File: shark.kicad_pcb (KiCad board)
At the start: 2 copper layers, 225.6 x 74.8 mm, 259 parts, among them J1 USB_C_Receptacle, Q1 AO4406AL, SW1 MXSwitch, SW10 MXSwitch, SW11 MXSwitch, SW12 MXSwitch, SW13 MXSwitch, SW14 MXSwitch, SW15 MXSwitch, SW16 MXSwitch, SW17 MXSwitch, SW18 MXSwitch, SW19 MXSwitch, SW2 MXSwitch, SW20 MXSwitch, SW21 MXSwitch, SW22 MXSwitch, SW23 MXSwitch, SW24 MXSwitch, SW25 MXSwitch, SW26 MXSwitch, SW27 MXSwitch, SW28 MXSwitch, SW29 MXSwitch, SW3 MXSwitch, SW30 MXSwitch, SW31 MXSwitch, SW32 MXSwitch, SW33 MXSwitch, SW34 MXSwitch, SW35 MXSwitch, SW36 MXSwitch, SW37 MXSwitch, SW38 MXSwitch, SW39 MXSwitch, SW4 MXSwitch, SW40 MXSwitch, SW41 MXSwitch, SW42 MXSwitch, SW43 MXSwitch, SW44 MXSwitch, SW45 MXSwitch, SW46 MXSwitch, SW47 MXSwitch, SW48 MXSwitch, SW49 MXSwitch, SW5 MXSwitch, SW50 MXSwitch, SW51 MXSwitch, SW6 MXSwitch, SW7 MXSwitch, SW8 MXSwitch, SW9 MXSwitch, U1 STM32F303CCT7, U2 MCP1700-3302E_SOT23, Y1 8MHz

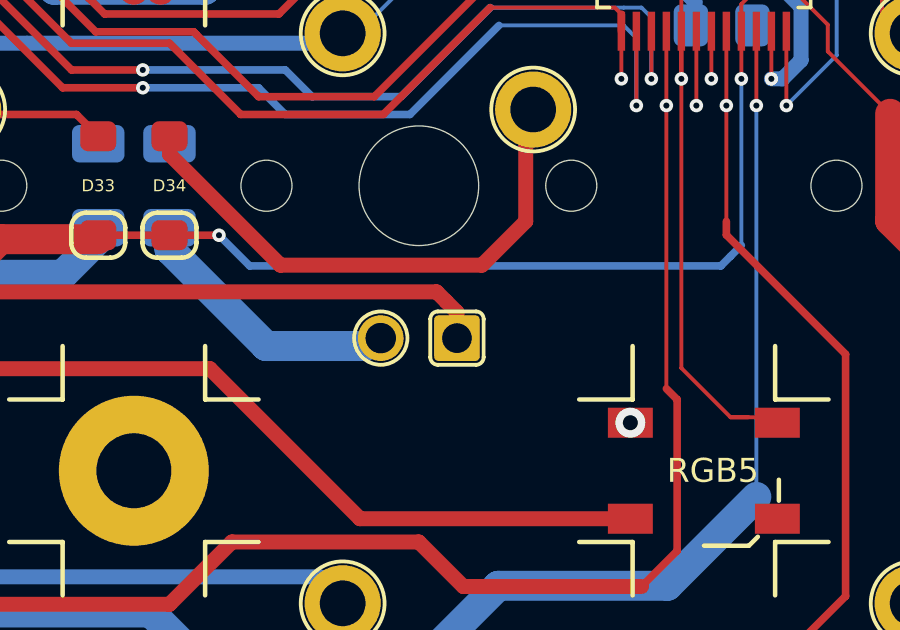
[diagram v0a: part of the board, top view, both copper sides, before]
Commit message: Edited gerbers
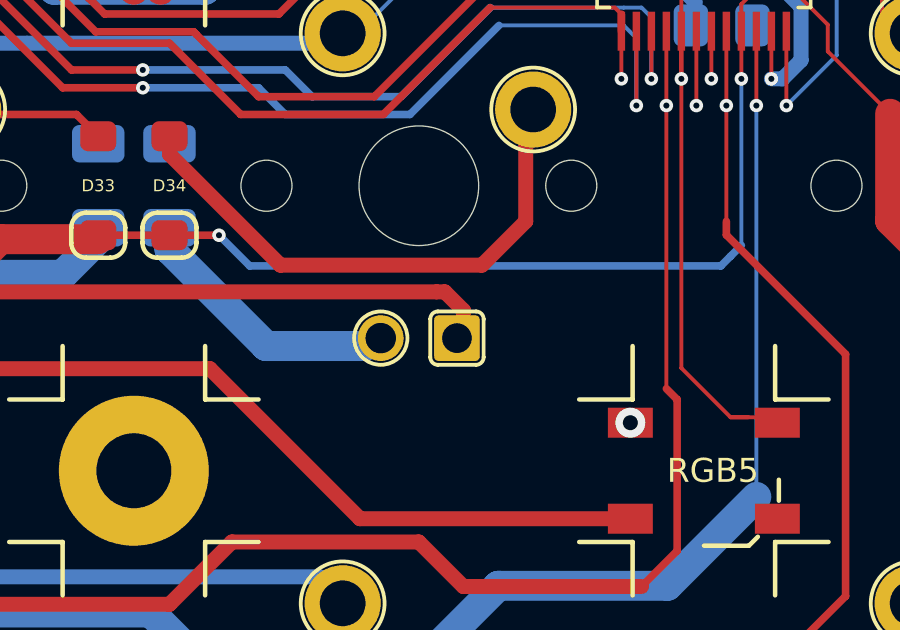
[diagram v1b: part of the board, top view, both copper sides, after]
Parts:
- removed the Y1 at (207.2, 102.4) (x2)
- added Y1 (x2): 8MHz, crystal:Crystal_SMD_5032-4Pin_5.0x3.2mm, F.Cu at (207.2, 102.4)
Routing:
- net Net-(LED1-PadK): track 1132.7 -> 1131.8 mm
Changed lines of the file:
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@@
     (thickness 1.6)
     (drawings 440)
-    (tracks 1809)
+    (tracks 1808)
     (zones 0)
     (modules 259)
@@
   (segment (start 64.1505 78.696125) (end 64.1505 78.993) (width 0.254) (layer F.Cu) (net 72) (status 30))
   (segment (start 197.1505 115.8055) (end 197.1505 116.696125) (width 0.5) (layer F.Cu) (net 72) (status 20))
-  (segment (start 216.233 117.323) (end 216.233 116.461) (width 0.5) (layer F.Cu) (net 72) (status 10))
   (segment (start 159.1505 116.993) (end 158.853625 116.993) (width 0.254) (layer F.Cu) (net 72) (status 30))
   (segment (start 235.233 117.323) (end 246.168 117.323) (width 1) (layer F.Cu) (net 72) (status 10))
@@
   (segment (start 121.12233 104.676825) (end 121.12233 100.990575) (width 1) (layer B.Cu) (net 72) (status 30))
   (via (at 121.39108 104.676825) (size 1) (drill 0.5) (layers F.Cu B.Cu) (net 72) (status 30))
-  (segment (start 216.233 117.323) (end 216.233 116.461) (width 0.254) (layer B.Cu) (net 72) (status 10))
   (segment (start 245.24425 131.243) (end 241.68175 131.243) (width 0.254) (layer F.Cu) (net 72))
   (segment (start 241.68175 131.243) (end 239.30675 133.618) (width 0.254) (layer F.Cu) (net 72))
@@
   (segment (start 135.4005 99.77425) (end 139.853625 99.77425) (width 0.7) (layer F.Cu) (net 72))
   (segment (start 133.94925 98.323) (end 135.4005 99.77425) (width 0.7) (layer F.Cu) (net 72))
-  (segment (start 216.233 116.461) (end 215.874375 116.102375) (width 0.5) (layer F.Cu) (net 72))
   (segment (start 159.1505 115.78125) (end 159.1505 117.289875) (width 0.5) (layer F.Cu) (net 72) (status 20))
   (segment (start 141.882 115.78125) (end 159.1505 115.78125) (width 0.5) (layer F.Cu) (net 72))
@@
   (segment (start 65.021073 137.111073) (end 65.021073 137.136198) (width 0.254) (layer F.Cu) (net 72))
   (segment (start 85.228625 100.071125) (end 102.125 100.071125) (width 0.7) (layer F.Cu) (net 72))
-  (segment (start 215.55325 115.78125) (end 215.874375 116.102375) (width 0.5) (layer F.Cu) (net 72))
   (segment (start 120.259875 100.071125) (end 121.1505 99.1805) (width 0.7) (layer F.Cu) (net 72))
   (segment (start 178.233 117.34747) (end 178.233 115.80572) (width 0.5) (layer F.Cu) (net 72))
   (segment (start 159.1505 115.78125) (end 178.233 115.78125) (width 0.5) (layer F.Cu) (net 72))
   (segment (start 178.233 115.78125) (end 215.55325 115.78125) (width 0.5) (layer F.Cu) (net 72))
+  (segment (start 215.55325 115.78125) (end 215.83029 115.78125) (width 0.5) (layer F.Cu) (net 72))
+  (segment (start 215.83029 115.78125) (end 216.44852 116.39948) (width 0.5) (layer F.Cu) (net 72))
+  (segment (start 216.44852 116.39948) (end 216.44852 116.99324) (width 0.5) (layer F.Cu) (net 72))
   (segment (start 55.24425 76.368) (end 58.463 79.58675) (width 1) (layer B.Cu) (net 73))
   (segment (start 55.24425 75.643) (end 55.24425 76.368) (width 1) (layer B.Cu) (net 73) (status 10))

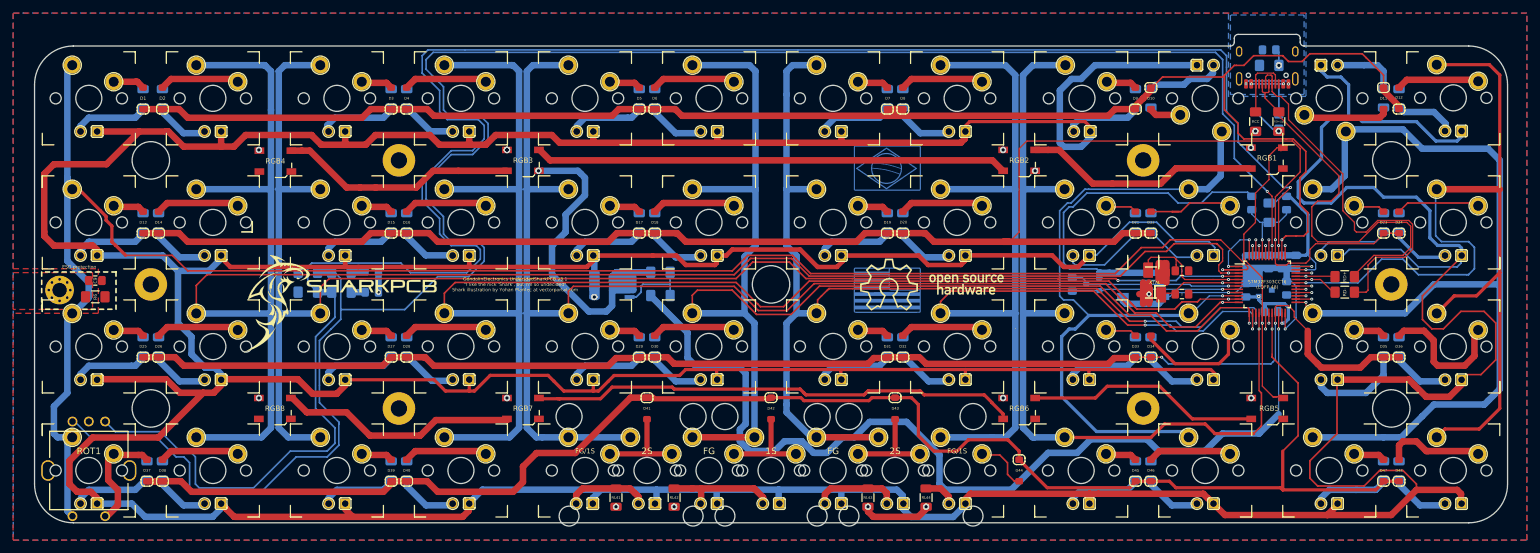
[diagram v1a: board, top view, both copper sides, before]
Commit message: Fixed little problem with edge cuts
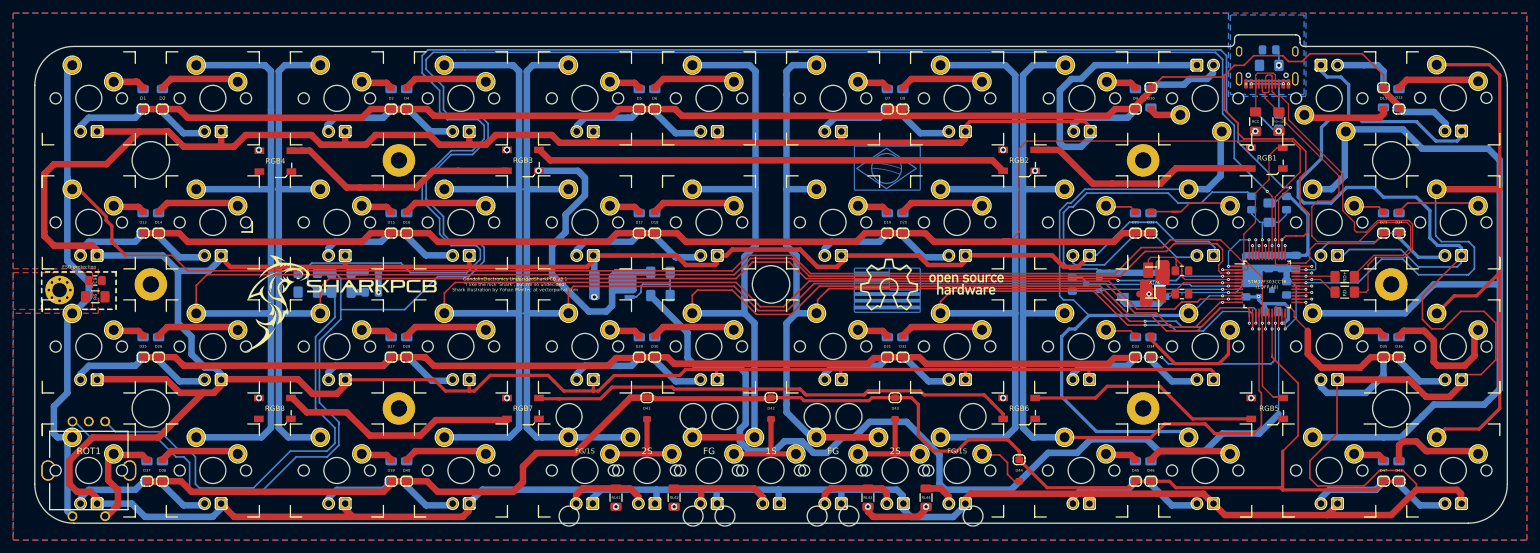
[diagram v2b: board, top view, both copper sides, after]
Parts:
- removed the Y1 at (207.2, 102.4) (x2)
- added Y1 (x2): 8MHz, crystal:Crystal_SMD_5032-4Pin_5.0x3.2mm, F.Cu at (207.2, 102.4)
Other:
- outline, holes or cut-outs redrawn
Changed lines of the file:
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@@
   (title_block
     (title SharkPCB)
-    (date 2019-02-20)
-    (rev V3.1)
+    (date 2019-02-27)
+    (rev V3.1.1)
     (company "Gondolin Electronics")
   )
@@
     )
   )
+  (gr_arc (start 255.27 72.263) (end 261.239 72.263) (angle -90) (layer Edge.Cuts) (width 0.15))
+  (gr_arc (start 230.124 65.659) (end 229.489 65.659) (angle -90) (layer Edge.Cuts) (width 0.15))
+  (gr_arc (start 228.854 65.151) (end 229.489 65.151) (angle -90) (layer Edge.Cuts) (width 0.15))
+  (gr_arc (start 220.091 65.151) (end 220.091 64.516) (angle -90) (layer Edge.Cuts) (width 0.15))
+  (gr_arc (start 218.821 65.659) (end 218.821 66.294) (angle -90) (layer Edge.Cuts) (width 0.15))
+  (gr_arc (start 41.656 72.263) (end 41.656 66.294) (angle -90) (layer Edge.Cuts) (width 0.15))
+  (gr_arc (start 41.656 133.35) (end 35.687 133.35) (angle -90) (layer Edge.Cuts) (width 0.15))
   (gr_text FG/1S (at 176.963 128.27425) (layer F.SilkS)
     (effects (font (size 0.75 0.75) (thickness 0.1875)))
@@
     (effects (font (size 0.8 0.8) (thickness 0.2)) (justify mirror))
   )
-  (gr_arc (start 41.588 72.164751) (end 41.588 66.227251) (angle -90) (layer Edge.Cuts) (width 0.15))
-  (gr_arc (start 41.588 133.321125) (end 35.6505 133.321125) (angle -90) (layer Edge.Cuts) (width 0.15))
-  (gr_arc (start 255.338 133.321125) (end 255.338 139.258625) (angle -90) (layer Edge.Cuts) (width 0.15))
-  (gr_arc (start 255.338 72.164875) (end 261.2755 72.164875) (angle -90) (layer Edge.Cuts) (width 0.15))
+  (gr_arc (start 255.27 133.35) (end 255.27 139.319) (angle -90) (layer Edge.Cuts) (width 0.15))
   (gr_circle (center 243.46332 121.743064) (end 246.330134 121.743064) (layer Edge.Cuts) (width 0.15))
   (gr_circle (center 243.46332 83.742936) (end 246.330134 83.742936) (layer Edge.Cuts) (width 0.15))
@@
   (gr_line (start 49.30675 67.118) (end 51.088 67.118) (layer F.SilkS) (width 0.15))
   (gr_line (start 51.088 67.118) (end 51.088 68.89925) (layer F.SilkS) (width 0.15))
-  (gr_line (start 220.009875 64.446125) (end 228.916396 64.445995) (layer Edge.Cuts) (width 0.15))
-  (gr_line (start 219.416125 65.633625) (end 219.416125 65.039875) (layer Edge.Cuts) (width 0.15))
-  (gr_arc (start 228.916398 65.039747) (end 229.510148 65.039747) (angle -90) (layer Edge.Cuts) (width 0.15))
-  (gr_arc (start 230.103623 65.633625) (end 229.509873 65.633625) (angle -90) (layer Edge.Cuts) (width 0.15))
-  (gr_arc (start 220.009875 65.039875) (end 220.009875 64.446125) (angle -90) (layer Edge.Cuts) (width 0.15))
-  (gr_arc (start 218.822612 65.633501) (end 218.822612 66.227251) (angle -90) (layer Edge.Cuts) (width 0.15))
+  (gr_line (start 220.091 64.516) (end 228.854 64.516) (layer Edge.Cuts) (width 0.15))
+  (gr_line (start 219.456 65.659) (end 219.456 65.151) (layer Edge.Cuts) (width 0.15))
   (gr_line (start 68.988926 93.118786) (end 68.988926 94.706286) (layer F.SilkS) (width 0.254))
   (gr_line (start 68.988926 94.706286) (end 67.401426 94.706286) (layer F.SilkS) (width 0.254))
-  (gr_line (start 229.509873 65.633625) (end 229.509873 65.039875) (layer Edge.Cuts) (width 0.15))
+  (gr_line (start 229.489 65.659) (end 229.489 65.151) (layer Edge.Cuts) (width 0.15))
   (gr_text "Surge\nprotection" (at 224.463 81.96175) (layer B.SilkS)
     (effects (font (size 0.508 0.508) (thickness 0.127)) (justify mirror))
@@
     (effects (font (size 0.508 0.508) (thickness 0.0762)))
   )
-  (gr_line (start 35.6505 133.321125) (end 35.6505 72.164875) (layer Edge.Cuts) (width 0.15))
-  (gr_line (start 255.338 139.258625) (end 41.588 139.258625) (layer Edge.Cuts) (width 0.15))
-  (gr_line (start 261.2755 72.164875) (end 261.2755 133.321125) (layer Edge.Cuts) (width 0.15))
+  (gr_line (start 35.687 133.35) (end 35.687 72.263) (layer Edge.Cuts) (width 0.15))
+  (gr_line (start 255.27 139.319) (end 41.656 139.319) (layer Edge.Cuts) (width 0.15))
+  (gr_line (start 261.239 72.263) (end 261.239 133.35) (layer Edge.Cuts) (width 0.15))
   (gr_text "GondolinElectronics UndecidedSharkPCB v3.1\n\"I like the nick 'Shark', but I'm so undecided\"\nShark illustration by Yohan Plantec at vectorportal.com" (at 109.2755 102.743) (layer F.SilkS)
     (effects (font (size 0.508 0.508) (thickness 0.0762)))
   )
-  (gr_line (start 230.103623 66.227375) (end 255.338 66.227375) (layer Edge.Cuts) (width 0.15))
-  (gr_line (start 41.588 66.227375) (end 218.822375 66.227375) (layer Edge.Cuts) (width 0.15))
+  (gr_line (start 230.124 66.294) (end 255.27 66.294) (layer Edge.Cuts) (width 0.15))
+  (gr_line (start 41.656 66.294) (end 218.821 66.294) (layer Edge.Cuts) (width 0.15))
   (segment (start 224.213 107.093) (end 224.213 109.571125) (width 0.13) (layer F.Cu) (net 0) (status 10))
   (segment (start 228.813 103.993) (end 231.291125 103.993) (width 0.13) (layer F.Cu) (net 0) (status 10))
